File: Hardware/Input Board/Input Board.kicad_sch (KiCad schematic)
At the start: 30 parts, among them J1 Relay, J10 Y Limit, J11 Z Limit, J12 Probe, J13 A Input, J14 Z Input, J15 Y Input, J16 X Input, J17 X Output, J18 Y Output, J19 Z Output, J2 24V, J20 A Output, J3 LED Lights, J4 Mist, J5 Motor Board, J6 Encoder Input, J7 Accessory, J8 Encoder Output, J9 X Limit, K1 SRD-24VDC-SL-C, K2 SRD-24VDC-SL-C

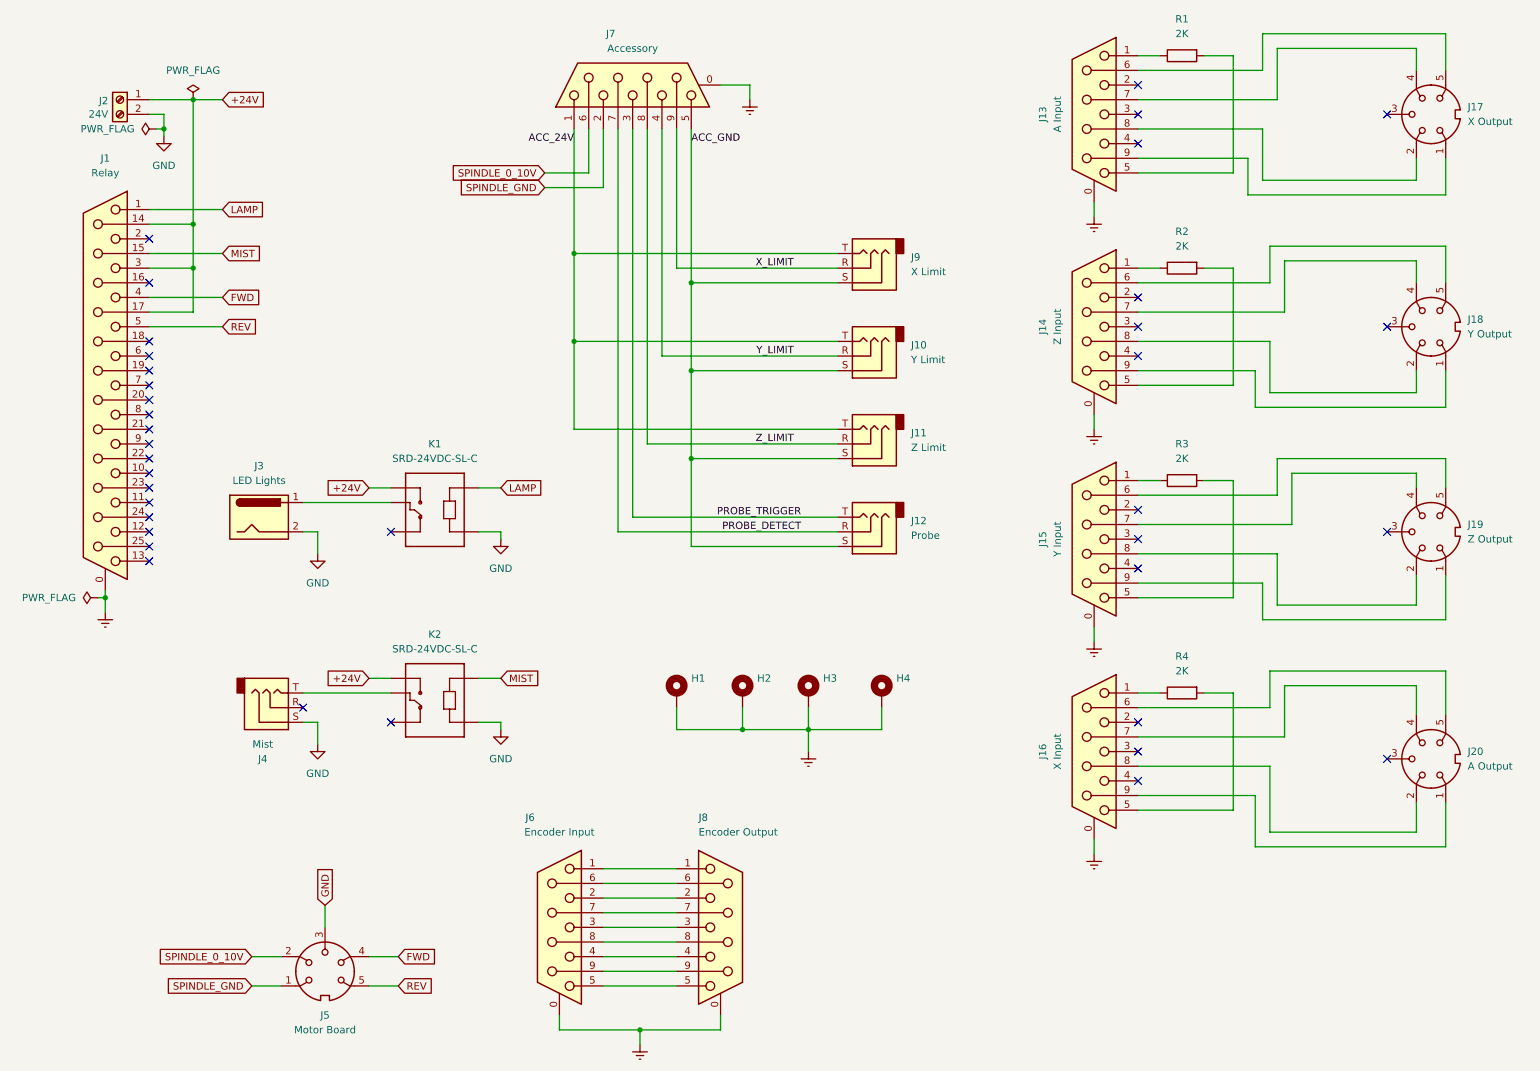
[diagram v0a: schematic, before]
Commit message: Library cleanup
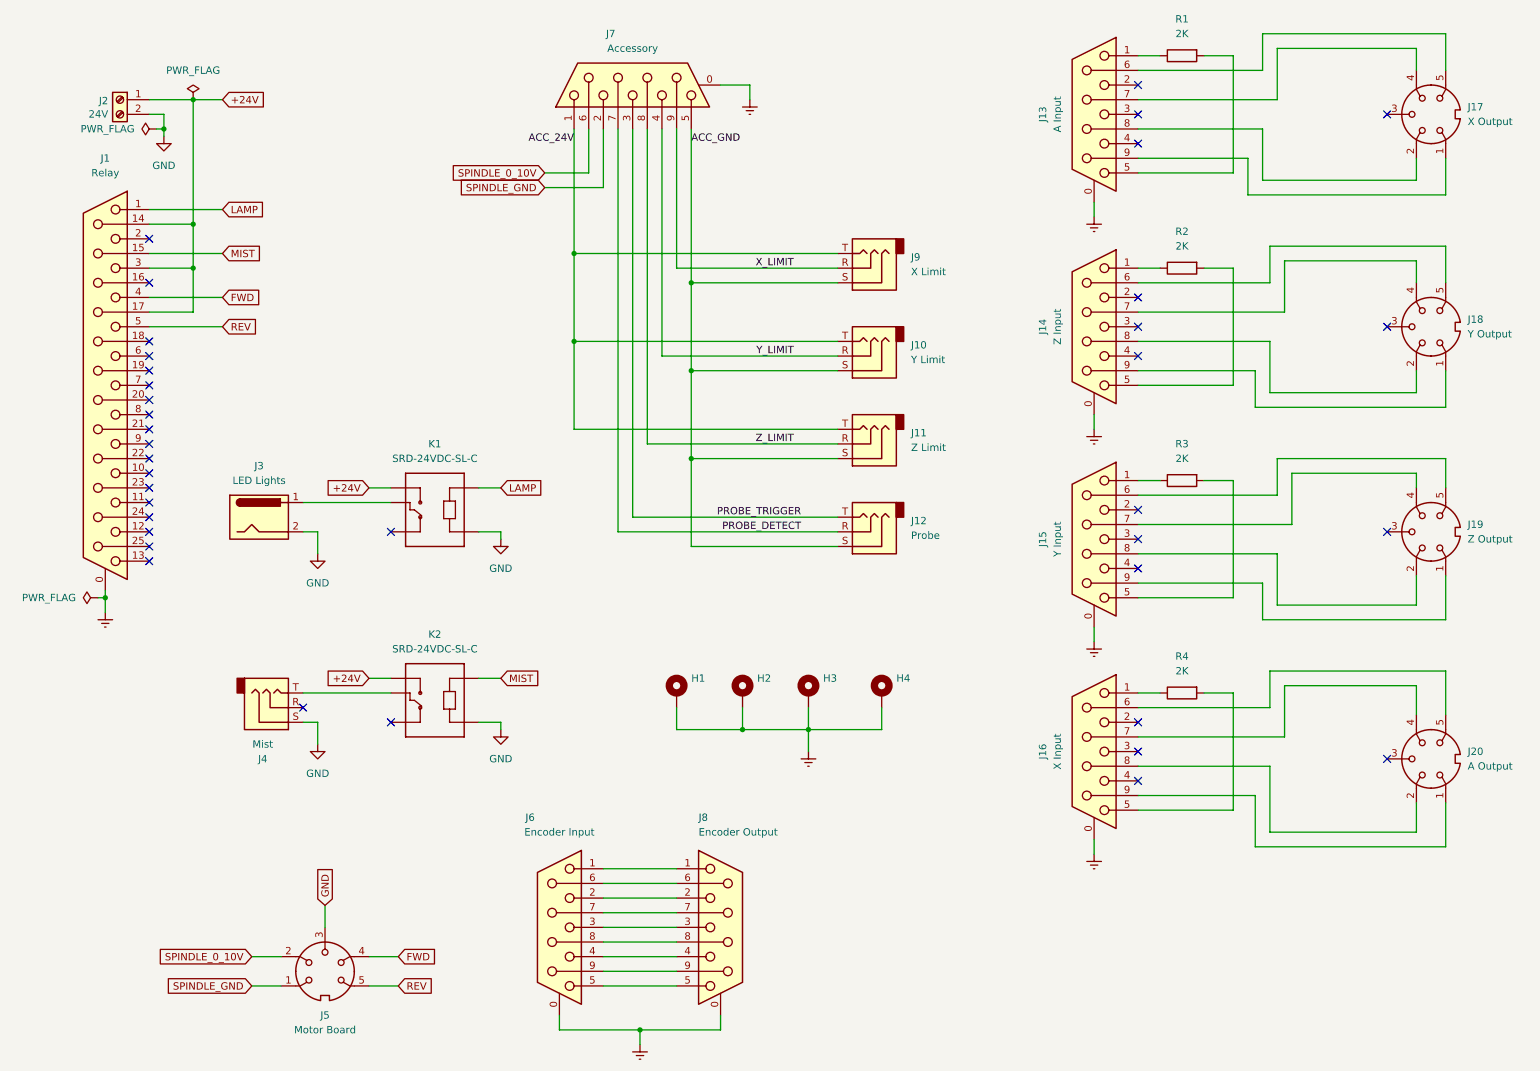
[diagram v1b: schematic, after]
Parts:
- H1, H2, H3, H4: footprint (none) -> MountingHole:MountingHole_3.2mm_M3
- J1: footprint (none) -> Connector_Dsub:DSUB-25_Female_Vertical_P2.77x2.84mm_MountingHoles
- J13, J14, J15, J16, J6, J7: footprint (none) -> Connector_Dsub:DSUB-9_Female_Vertical_P2.77x2.84mm_MountingHoles
- J17, J18, J19, J20, J5: footprint (none) -> DIN5-RA-PTH:DIN5-RA-PTH
- J2: footprint (none) -> TerminalBlock_Phoenix:TerminalBlock_Phoenix_PT-1,5-2-5.0-H_1x02_P5.00mm_Horizontal
- J3: footprint (none) -> Connector_BarrelJack:BarrelJack_Horizontal
- J8: footprint (none) -> Connector_Dsub:DSUB-9_Female_Horizontal_P2.77x2.84mm_EdgePinOffset9.90mm_Housed_MountingHolesOffset11.32mm
- K1, K2: footprint Input Board:SRD-24VDC-SL-C -> SRD-24VDC-SL-C:SRD-24VDC-SL-C
- R1, R2, R3, R4: footprint (none) -> Resistor_THT:R_Axial_DIN0411_L9.9mm_D3.6mm_P15.24mm_Horizontal
